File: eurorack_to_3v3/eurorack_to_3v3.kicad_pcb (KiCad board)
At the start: 2 copper layers, 47.5 x 96 mm, 138 parts, among them J1 cv_in_2, J2 gate_in_2, J3 gate_in_1, J4 cv_in_1, J5 Eurorack Power Header, J6 Brain Bus, J7 gate_in_3, J8 gate_out, J9 cv_out, U1 MCP3208, U10 MOSFET_RK7002BM, U11 MOSFET_RK7002BM, U12 MOSFET_RK7002BM, U13 MOSFET_RK7002BM, U14 MOSFET_RK7002BM, U15 MOSFET_RK7002BM, U16 MOSFET_RK7002BM, U17 MOSFET_RK7002BM, U18 MOSFET_RK7002BM, U19 MOSFET_RK7002BM, U2 74HC589, U20 MOSFET_RK7002BM, U21 MOSFET_RK7002BM, U23 TL074CDT, U24 LM324, U3 LM324, U4 74HC589, U5 74HC137, U6 BH2227FV, U7 74HC595, U8 MCP6009, U9 MCP6009

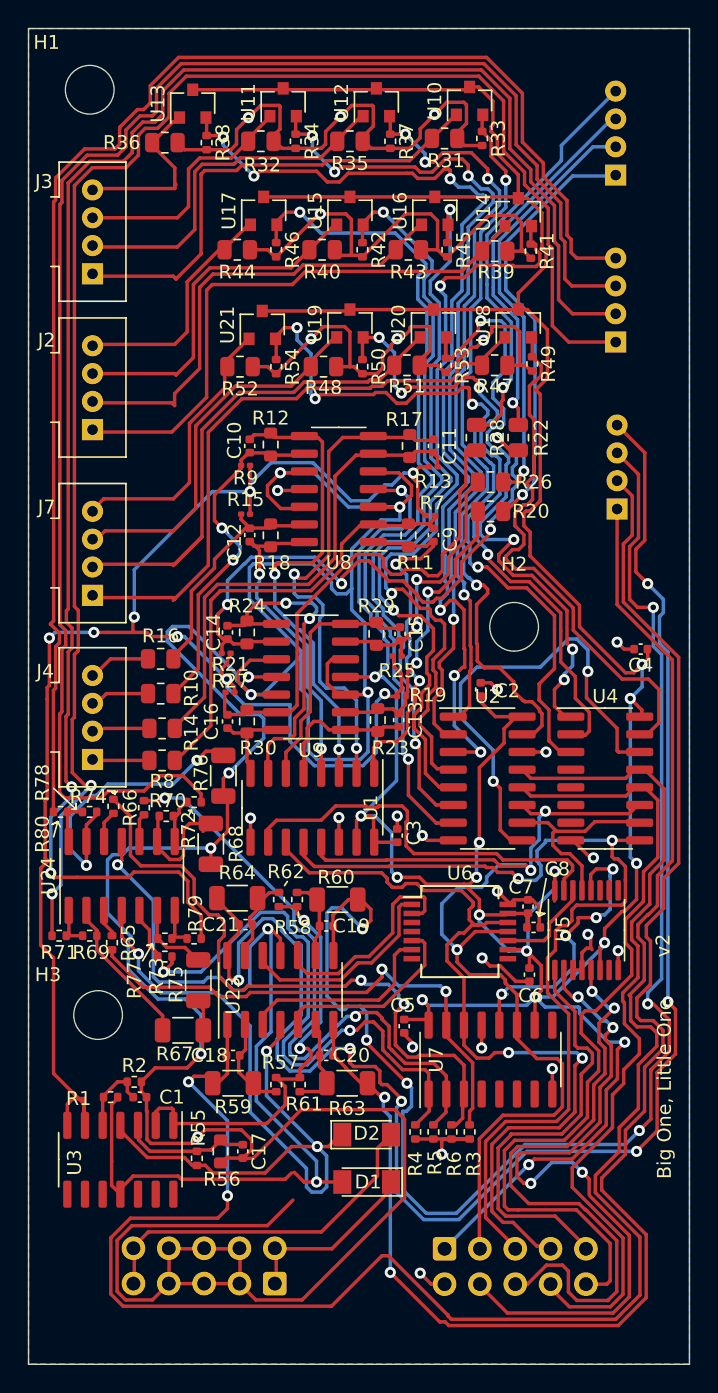
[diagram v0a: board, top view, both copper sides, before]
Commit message: cleanup tracks
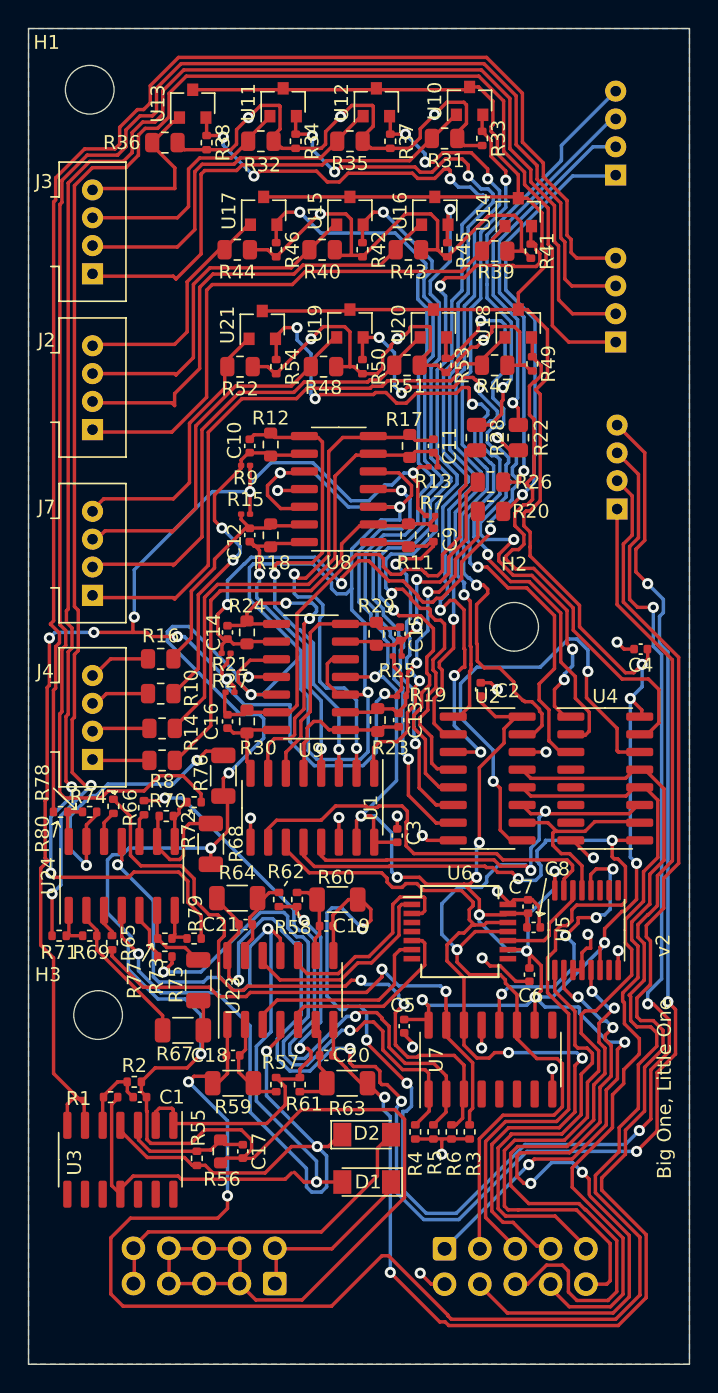
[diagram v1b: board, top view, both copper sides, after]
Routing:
- net GND: track 241.1 -> 219.2 mm, vias 8 -> 7
- net /gate_to_3v3_C/GATE_IN_2: track 37.3 -> 34.6 mm
- net GNDD: track 153.1 -> 150.9 mm
- net +3V3: track 281.2 -> 279.9 mm
- net Net-(C21-Pad2): track 7.54 -> 6.33 mm
- net /AREF_-10V: track 120.9 -> 119.8 mm
- net /GATE_IN_EN: track 15.3 -> 14.4 mm
- net Net-(R68-Pad1): track 9.33 -> 8.53 mm
- net /gate_to_3v3_C/GATE_IN_1: track 43.9 -> 43.2 mm
- net /3v3_to_cv/CV_3V3_4: track 15.7 -> 15.1 mm
